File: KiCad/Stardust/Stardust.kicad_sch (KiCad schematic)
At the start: 10 parts, among them IC1 TS1117BCW50_RPG, J1 Jack-DC, J2 85513-5002, U1 ESP32-DEVKITC, U2 TMC2209_SILENTSTEPSTICK, U3 TMC2209_SILENTSTEPSTICK, U4 WEMOS_D1_mini, U5 RTC 3013, U6 MC7812BDTRKG, U7 56200001009

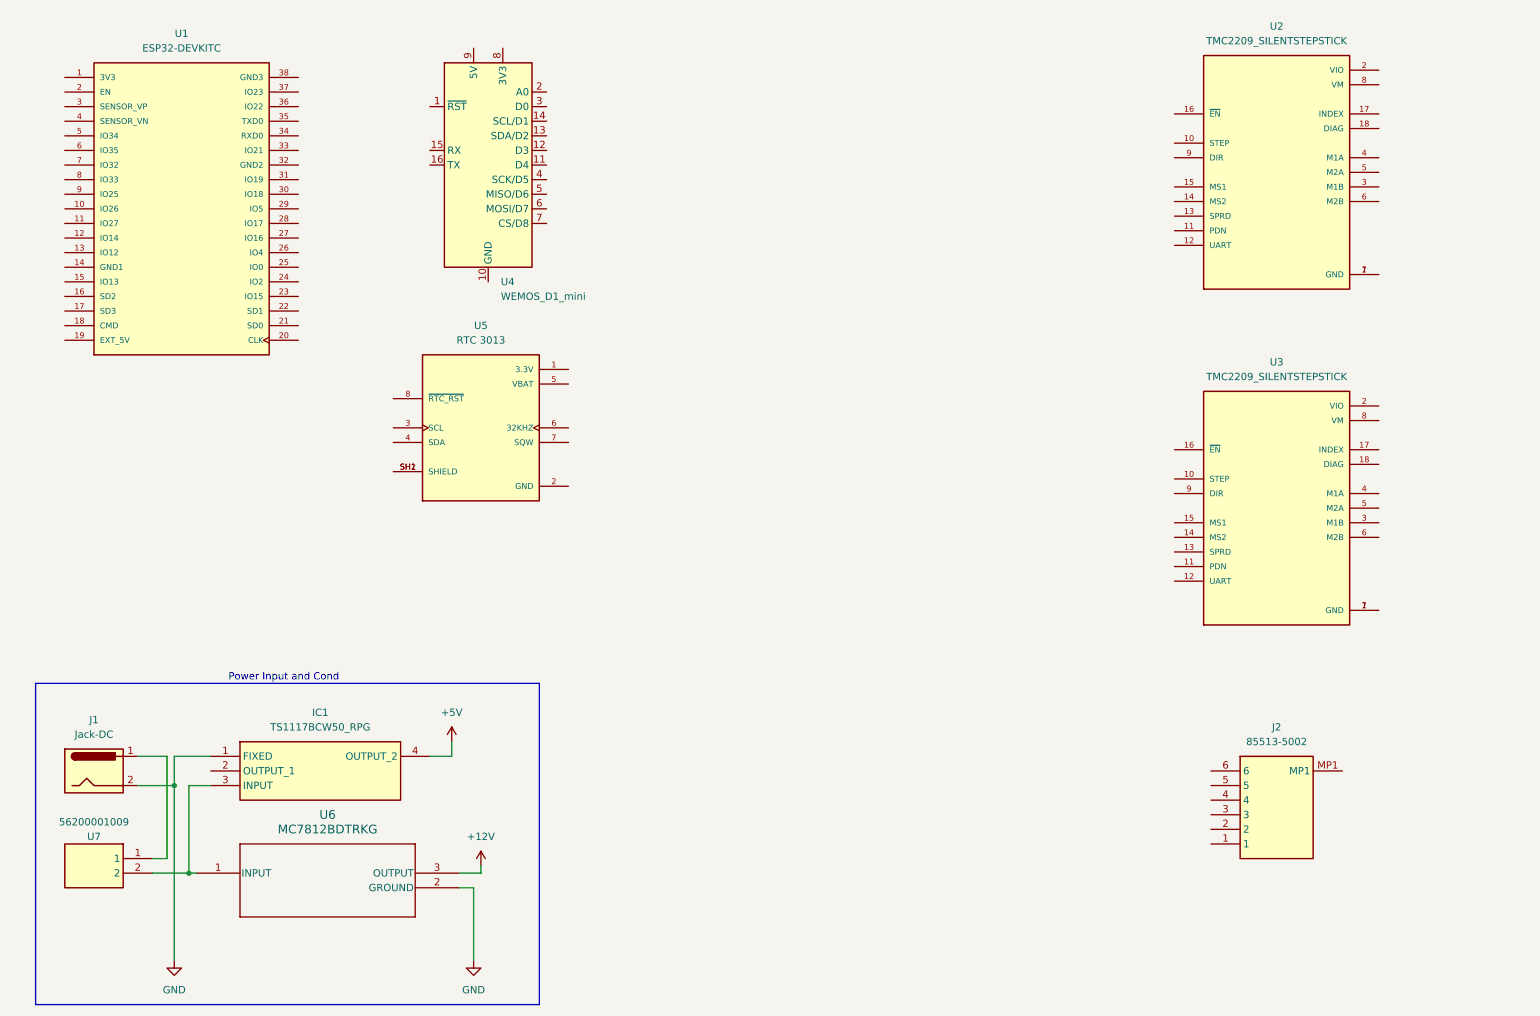
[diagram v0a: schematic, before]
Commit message: Finished schematic (V1.0)
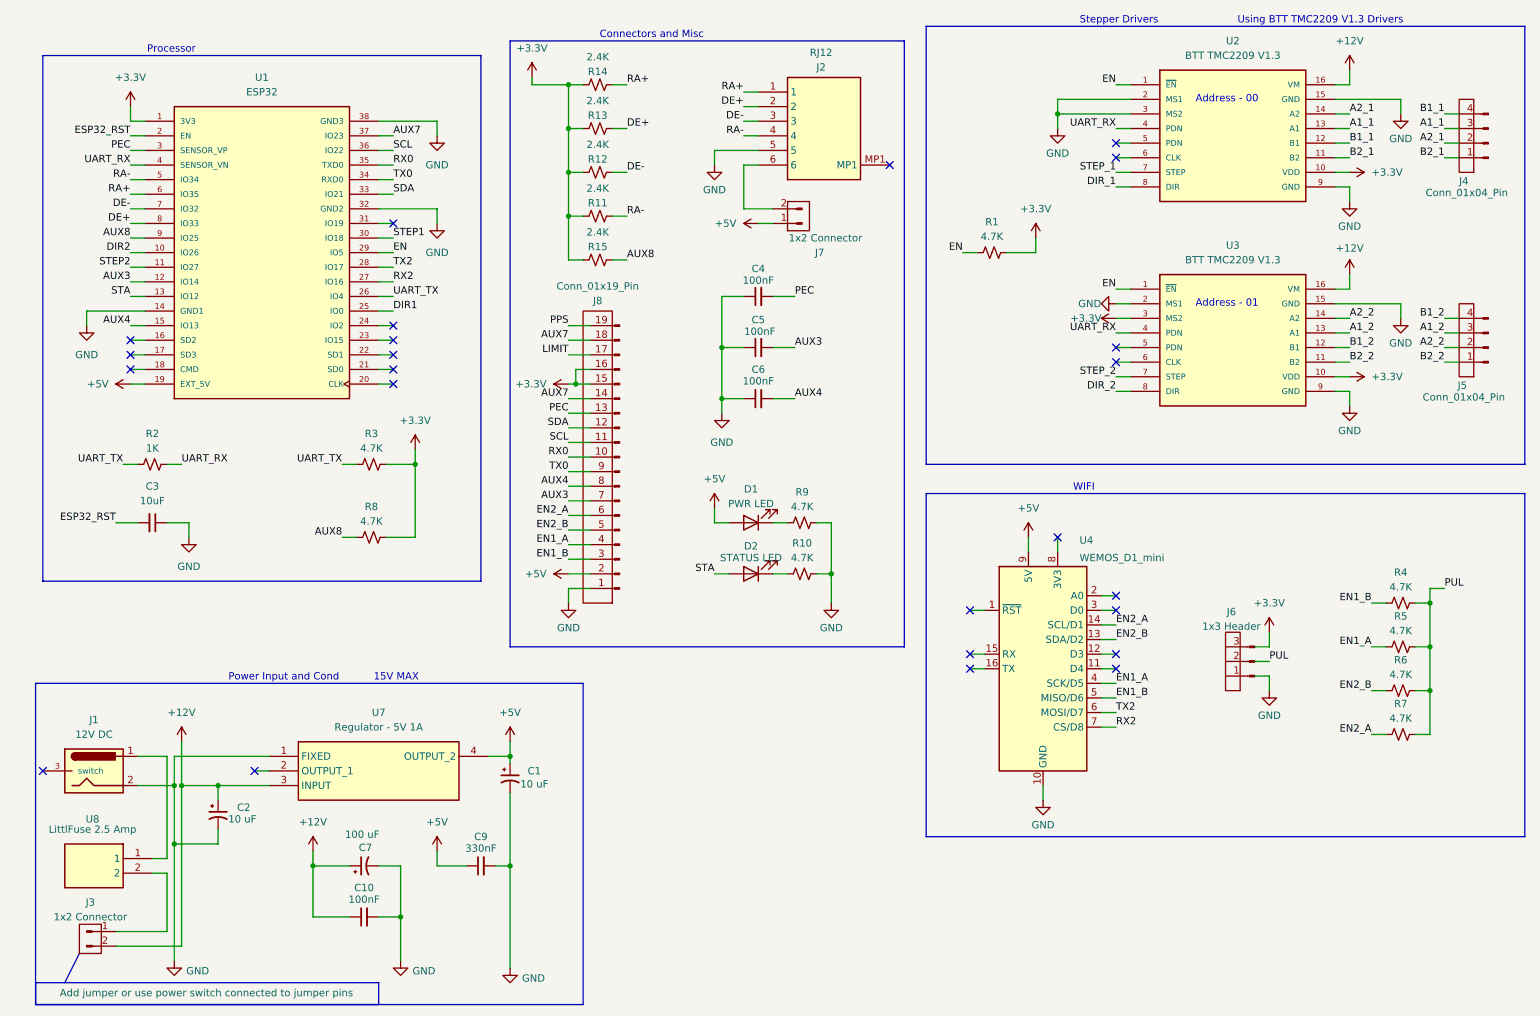
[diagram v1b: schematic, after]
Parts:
- removed U5: RTC 3013, Stardust:MODULE_3013, symbol RTC:3013
- removed U6: MC7812BDTRKG, Stardust:12VREG_DPAK-3_ONS, symbol 12V Regulator:MC7812BDTRKG
- added C1, C2: 10 uF, symbol Device:C_Polarized_Small_US
- added C10, C4, C5, C6: 100nF, symbol Device:C_Small
- added C3: 10uF, symbol Device:C_Small
- added C7: 100 uF, symbol Device:C_Polarized_Small_US
- added C9: 330nF, symbol Device:C_Small
- added D1: PWR LED, symbol Device:LED
- added D2: STATUS LED, symbol Device:LED
- added J3, J7: 1x2 Connector, Connector_PinHeader_2.54mm:PinHeader_1x02_P2.54mm_Vertical, symbol Connector:Conn_01x02_Pin
- added J4, J5: Conn_01x04_Pin, symbol Connector:Conn_01x04_Pin
- added J6: 1x3 Header, symbol Connector:Conn_01x03_Pin
- added J8: Conn_01x19_Pin, symbol Connector:Conn_01x19_Pin
- added R1, R10, R3, R4, R5, R6, R7, R8, R9: 4.7K, Resistor_SMD:R_0402_1005Metric, symbol Device:R_Small_US
- added R11, R12, R13, R14, R15: 2.4K, Resistor_SMD:R_0402_1005Metric, symbol Device:R_Small_US
- added R2: 1K, Resistor_SMD:R_0402_1005Metric, symbol Device:R_Small_US
- J1: value Jack-DC -> 12V DC
- J2: value 85513-5002 -> RJ12
- U1: value ESP32-DEVKITC -> ESP32; Availability Not in stock -> (none); Check_prices https://www.snapeda.com/parts/ESP32-DEVKITC/Espressif+Syste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 -> (none); Description_1 ESP32-WROOM-32UE series Transceiver; 802.11 b/g/n (Wi-Fi, W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 -> (none); Link (none) -> https://www.digikey.com/en/products/detail/espressif-system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; MANUFACTURER ESPRESSIF -> (none); MP ESP32-DEVKITC -> (none); PARTREV N/A -> (none); Package None -> (none); Price None -> (none); STANDARD Manufacturer Recommendations -> (none); SnapEDA_Link https://www.snapeda.com/parts/ESP32-DEVKITC/Espressif+Syste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 -> (none)
- U2, U3: value TMC2209_SILENTSTEPSTICK -> BTT TMC2209 V1.3; Availability Not in stock -> (none); Check_prices https://www.snapeda.com/parts/TMC2209%20SILENTSTEPSTICK/Tri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 -> (none); Description_1 TMC2209 Motor Controller/Driver Power Management Evaluation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 -> (none); MANUFACTURER Trinamic Motion Control GmbH -> (none); MF Trinamic Motion Control GmbH -> BIGTREETECH; MP TMC2209 SILENTSTEPSTICK -> (none); PARTREV 1.20 -> (none); Package None -> (none); Price None -> (none); SNAPEDA_PN TMC2209 SILENTSTEPSTICK -> (none); STANDARD Manufacturer Recommendations -> (none); SnapEDA_Link https://www.snapeda.com/parts/TMC2209%20SILENTSTEPSTICK/Tri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 -> (none)
- U7: renamed from IC1; value TS1117BCW50_RPG -> Regulator - 5V 1A
- U8: renamed from U7; value 56200001009 -> LittlFuse 2.5 Amp
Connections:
- net +12V: now also U2.16 (VM), U3.16 (VM), U7.3 (INPUT), C10.1, C2.1, C7.1, J3.2 (Pin_2)
- net +5V: now also U1.19 (EXT_5V), U4.9 (5V), C1.1, C9.1, D1.2 (A), J7.1 (Pin_1), J8.2 (Pin_2)
- net GND: now also J2.5, U1.14 (GND1), U1.32 (GND2), U1.38 (GND3), U2.15 (GND), U2.2 (MS1), U2.3 (MS2), U2.9 (GND), U3.15 (GND), U3.2 (MS1), U3.9 (GND), U4.10 (GND), C1.2, C10.2, C2.2, C3.1, C4.1, C5.1, C6.1, C7.2, C9.2, J8.1 (Pin_1), R10.2, R9.2
- net at U8.2: now also J3.1 (Pin_1); no longer U7.3 (INPUT)
- net EN: now reaches U2.1 (~{EN})
- net EN: now also U1.29 (IO5), U3.1 (~{EN}), R1.1; no longer U2.7 (GND)
- net +3.3V: now reaches U2.10 (VDD)
- net +3.3V: now also U1.1 (3V3), U3.10 (VDD), U3.3 (MS2), J8.15 (Pin_15), J8.16 (Pin_16), R1.2, R11.2, R12.2, R13.2, R14.2, R15.2, R3.2, R8.2
- net B2_1: now reaches U2.11 (B2)
- net B2_1: now also J4.1 (Pin_1)
- net B1_1: now reaches U2.12 (B1)
- net B1_1: now also J4.4 (Pin_4)
- net A1_1: now reaches U2.13 (A1)
- net A1_1: now also J4.3 (Pin_3)
- net A2_1: now reaches U2.14 (A2)
- net A2_1: now also J4.2 (Pin_2)
- net UART_RX: now reaches U2.4 (PDN)
- net UART_RX: now also U1.4 (SENSOR_VN), U3.4 (PDN), R2.2
- net DIR_1: now reaches U2.8 (DIR)
- net DIR2: now reaches U1.10 (IO26)
- net STEP2: now reaches U1.11 (IO27)
- net AUX3: now reaches U1.12 (IO14)
- net AUX3: now also C5.2, J8.7 (Pin_7)
- net STA: now reaches U1.13 (IO12)
- net STA: now also D2.2 (A)
- net AUX4: now reaches U1.15 (IO13)
- net AUX4: now also C6.2, J8.8 (Pin_8)
- net ESP32_RST: now reaches U1.2 (EN)
- net ESP32_RST: now also C3.2
- net DIR1: now reaches U1.25 (IO0)
- net UART_TX: now reaches U1.26 (IO4)
- net UART_TX: now also R2.1, R3.1
- net RX2: now reaches U1.27 (IO16)
- net RX2: now also U4.7 (CS/D8)
- net TX2: now reaches U1.28 (IO17)
- net TX2: now also U4.6 (MOSI/D7)
- net PEC: now reaches U1.3 (SENSOR_VP)
- net PEC: now also C4.2, J8.13 (Pin_13)
- net STEP1: now reaches U1.30 (IO18)
- net SDA: now reaches U1.33 (IO21)
- net SDA: now also J8.12 (Pin_12)
- net TX0: now reaches U1.34 (RXD0)
- net TX0: now also J8.9 (Pin_9)
- net RX0: now reaches U1.35 (TXD0)
- net RX0: now also J8.10 (Pin_10)
- net SCL: now reaches U1.36 (IO22)
- net SCL: now also J8.11 (Pin_11)
- net AUX7: now reaches U1.37 (IO23)
- net AUX7: now also J8.14 (Pin_14), J8.18 (Pin_18)
- net RA-: now reaches U1.5 (IO34)
- net RA-: now also J2.4, R11.1
- net RA+: now reaches U1.6 (IO35)
- net RA+: now also J2.1, R14.1
- net DE-: now reaches U1.7 (IO32)
- net DE-: now also J2.3, R12.1
- net DE+: now reaches U1.8 (IO33)
- net DE+: now also J2.2, R13.1
- net AUX8: now reaches U1.9 (IO25)
- net AUX8: now also R15.1, R8.1
- net STEP_2: now reaches U3.7 (STEP)
- net STEP_2: no longer U3.1 (GND)
- net B2_2: now reaches U3.11 (B2)
- net B2_2: now also J5.1 (Pin_1)
- net B1_2: now reaches U3.12 (B1)
- net B1_2: now also J5.4 (Pin_4)
- net A1_2: now reaches U3.13 (A1)
- net A1_2: now also J5.3 (Pin_3)
- net A2_2: now reaches U3.14 (A2)
- net A2_2: now also J5.2 (Pin_2)
- net DIR_2: now reaches U3.8 (DIR)
- net EN2_B: now reaches U4.13 (SDA/D2)
- net EN2_B: now also J8.5 (Pin_5), R6.1
- net EN2_A: now reaches U4.14 (SCL/D1)
- net EN2_A: now also J8.6 (Pin_6), R7.1
- net EN1_A: now reaches U4.4 (SCK/D5)
- net EN1_A: now also J8.4 (Pin_4), R5.1
- net EN1_B: now reaches U4.5 (MISO/D6)
- net EN1_B: now also J8.3 (Pin_3), R4.1
- net at J2.6: now also J7.2 (Pin_2)
- new net: D1.1 (K), R9.1
- new net: D2.1 (K), R10.1
- new net LIMIT: J8.17 (Pin_17)
- new net PPS: J8.19 (Pin_19)
- new net PUL: R4.2, R5.2, R6.2, R7.2
- new net STEP_1: U2.7 (STEP)
- no-connect marks 0 -> 24
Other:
- note added: "15V MAX"
- note added: "Address - 00"
- note added: "Address - 01"
- note added: "Connectors and Misc"
- note added: "Processor"
- note added: "Stepper Drivers"
- note added: "Using BTT TMC2209 V1.3 Drivers"
- note added: "WIFI"
- moved on the sheet: J2, U4, U7
